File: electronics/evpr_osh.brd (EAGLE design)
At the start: 93.2 x 42.7 mm, 140 parts

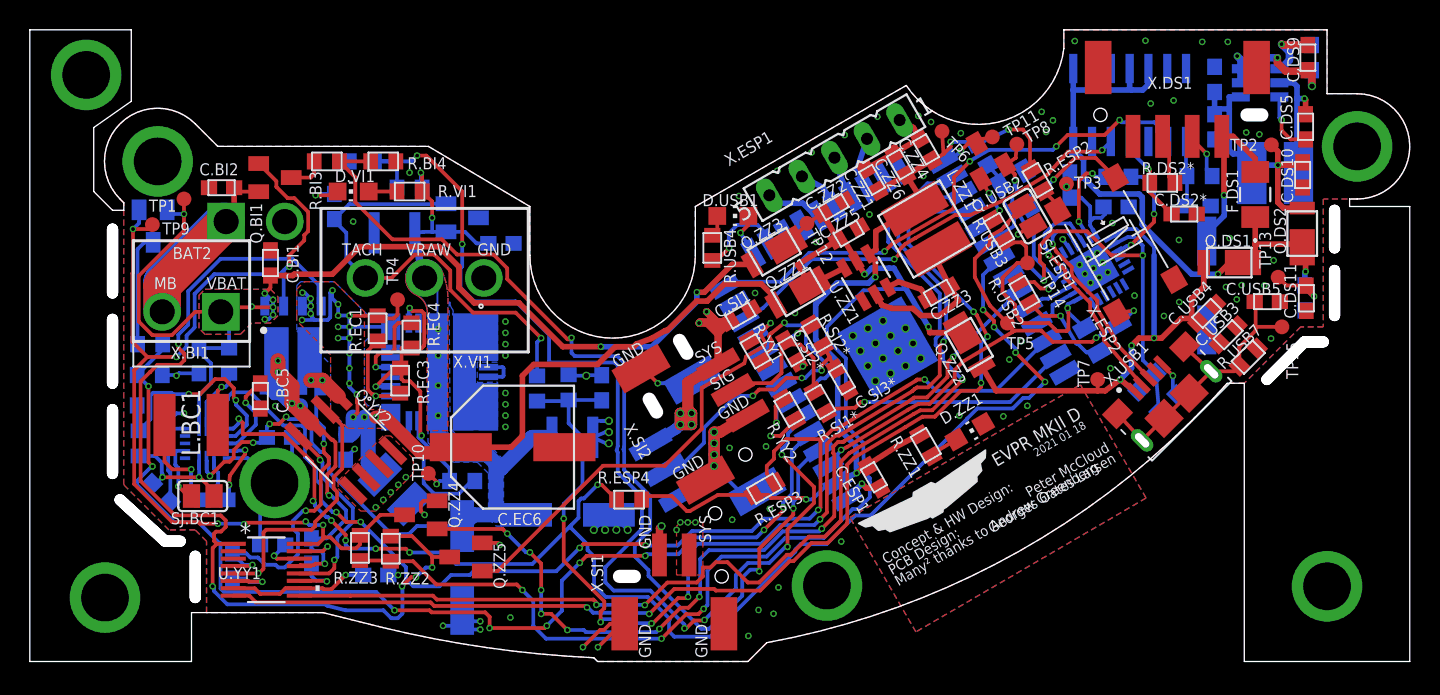
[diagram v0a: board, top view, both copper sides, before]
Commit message: Update osh version
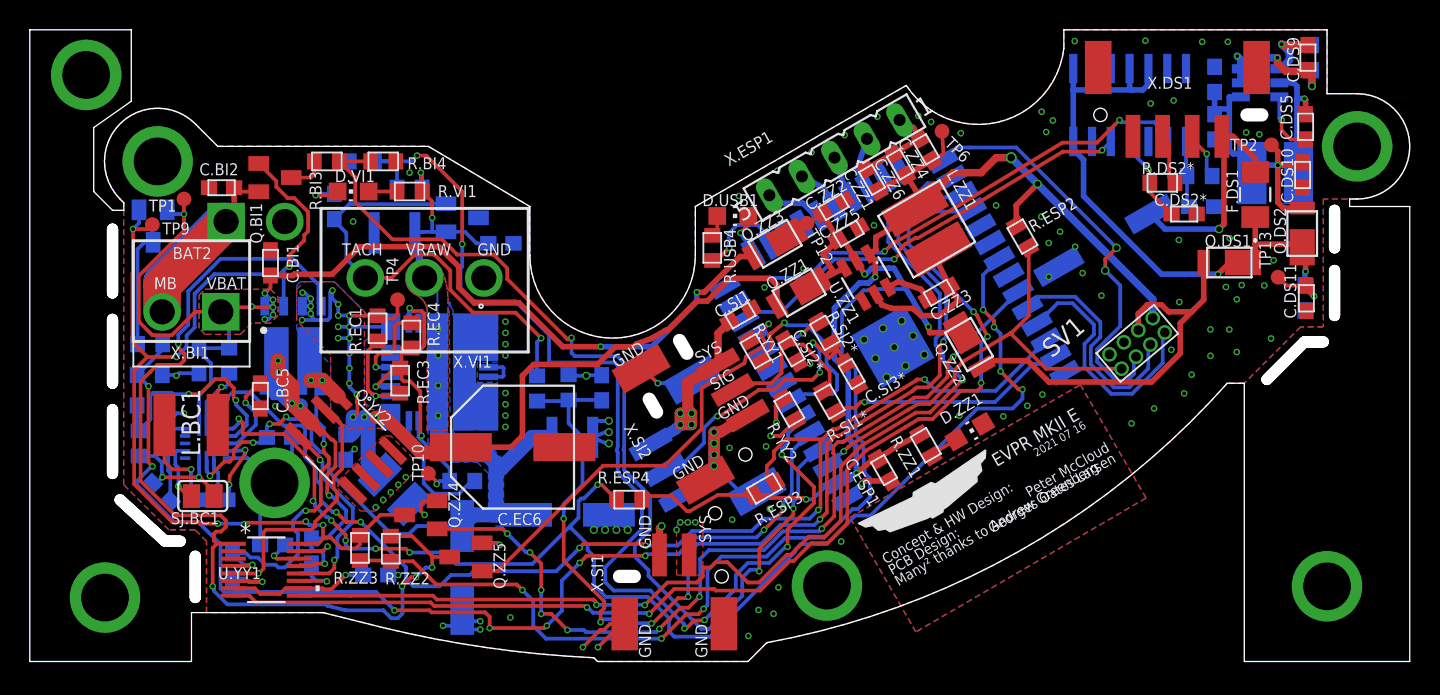
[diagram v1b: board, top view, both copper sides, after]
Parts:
- removed C.USB1, C.USB4: 4.7uF, mccloud:C0603
- removed C.USB2, C.USB3: 0.1uF, mccloud:C0603
- removed C.USB5: 4.7 nF, mccloud:C0603
- removed Q.ESP1: DMN5L06K-7, mccloud:SOT23
- removed Q.USB1, Q.USB2: MMBT2222A, transistor-neu-to92:SOT23-BEC
- removed R.ESP1, R.USB2, R.USB3: 10k, mccloud:R0603
- removed R.USB1: 1k, mccloud:R0603
- removed R.USB5: 22.1k, mccloud:R0603
- removed R.USB6: 47.5K, mccloud:R0603
- removed R.USB7: 1M, mccloud:R0603
- removed SJ.ESP1: (no value), jumper:SJ
- removed TP11, TP14, TP15, TP3, TP5, TP7, TP8: PTR1TP10R, testpad:TP10R
- removed U.USB1: CP2102N-A02-GQFN24R, mccloud:QFN24-4X4
- removed X.ESP2: RSTBTN, mccloud:PTS645
- removed X.USB1: 10118193-0001LF, mccloud:FCI_10118193-0001LF
- added SV1: PR20B04HBDN, mccloud:PR20B04HBDN
- moved C.DS1 7.55 mm to (33.2, -27.7), turned to 60 degrees
- moved R.ESP2 3.94 mm to (27.7, -27.4)
- moved C.ESP1 0.84 mm to (18.3, -43.2)
- moved C.SI3* 0.76 mm to (16.2, -36.7)
- moved R.SI1* 0.64 mm to (14.7, -38.6)
- moved R.SI2* 0.56 mm to (14.4, -33.9)
- moved Q.ZZ3 0.54 mm to (11.0, -27.9)
- moved C.DS4* 0.23 mm to (39.8, -25.4)
- moved Q.ZZ1 0.08 mm to (12.6, -31.2)
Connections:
- removed net N$1: Q.ESP1.3, X.ESP2.P$1, X.ESP2.P$2
- removed net N$16: R.USB1.1, U.USB1.9
- removed net N$18: Q.USB1.E, R.USB3.2, TP14.TP, U.USB1.19
- removed net N$19: Q.USB2.E, R.USB2.2, TP8.TP, U.USB1.23
- removed net N$20: Q.USB1.B, R.USB2.1
- removed net N$21: Q.USB2.B, R.USB3.1
- removed net N$34: C.USB5.2, R.USB7.2, TP15.TP, X.USB1.S1, X.USB1.S2, X.USB1.S3, X.USB1.S4, X.USB1.S5, X.USB1.S6
- removed net N$39: R.USB1.2, U.USB1.5
- removed net N$40: C.USB1.2, C.USB2.2, TP3.TP, U.USB1.6
- removed net RST_DISABLE: Q.ESP1.1, R.ESP1.2, U.ESP1.30
- removed net USBD+: U.USB1.3, X.USB1.3
- removed net USBD-: U.USB1.4, X.USB1.2
- removed net USBSENSE: R.USB5.1, R.USB6.2, U.ESP1.32, U.USB1.8
- removed net VUSB: C.USB3.2, C.USB4.2, Q.DS1.A, Q.ZZ2.A, R.USB5.2, TP7.TP, U.USB1.7, X.USB1.1
- new net VPROG: Q.DS1.A, Q.ZZ2.A, SV1.P$6
- net BOOTMODE: now also SV1.P$3; no longer Q.USB2.C, TP11.TP
- net ESP_POWER: now also SV1.P$8; no longer R.ESP1.1
- net ESP_RX: now also SV1.P$5; no longer U.USB1.21
- net ESP_TX: now also SV1.P$7; no longer U.USB1.20
- net GND: now also SV1.P$2; no longer C.USB1.1, C.USB2.1, C.USB3.1, C.USB4.1, C.USB5.1, Q.ESP1.2, R.USB6.1, R.USB7.1, SJ.ESP1.1, U.USB1.2, U.USB1.EXP, X.USB1.5
- net RESET: now also SV1.P$1; no longer Q.USB1.C, SJ.ESP1.2, TP5.TP, X.ESP2.P$3, X.ESP2.P$4
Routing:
- net VUSB: track 38.4 -> 0.00 mm, vias 3 -> 0
- net USBSENSE: track 27.4 -> 0.00 mm, vias 2 -> 0
- net VPROG: track 0.00 -> 26.9 mm
- net BOOTMODE: track 3.97 -> 28.4 mm, vias 1 -> 2
- net N$34: track 20.2 -> 0.00 mm
- net USBD-: track 16.3 -> 0.00 mm, vias 1 -> 0
- net N$18: track 16.1 -> 0.00 mm, vias 1 -> 0
- net N$19: track 14.8 -> 0.00 mm, vias 2 -> 0
- net ESP_POWER: track 63.6 -> 78.1 mm
- net USBD+: track 14.3 -> 0.00 mm, vias 1 -> 0
- net ESP_TX: track 3.57 -> 17.2 mm
- net ESP_RX: track 3.31 -> 15.8 mm
- net RESET: track 40.7 -> 30.6 mm, vias 3 -> 1
- net N$1: track 7.80 -> 0.00 mm, vias 1 -> 0
- net N$16: track 7.38 -> 0.00 mm, vias 2 -> 0
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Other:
- board text added: "2021 07 16"
- board text added: "EVPR MKII E"
- board text removed: "2021 01 18"
- board text removed: "EVPR MKII D"
